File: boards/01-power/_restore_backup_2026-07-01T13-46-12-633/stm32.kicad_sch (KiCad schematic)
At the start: 26 parts, among them J3 TC2030, SW1 SW_BOOT, SW2 SW_BOOT, SW3 SW_BOOT, U3 STM32F405RGTx, Y1 16Mhz

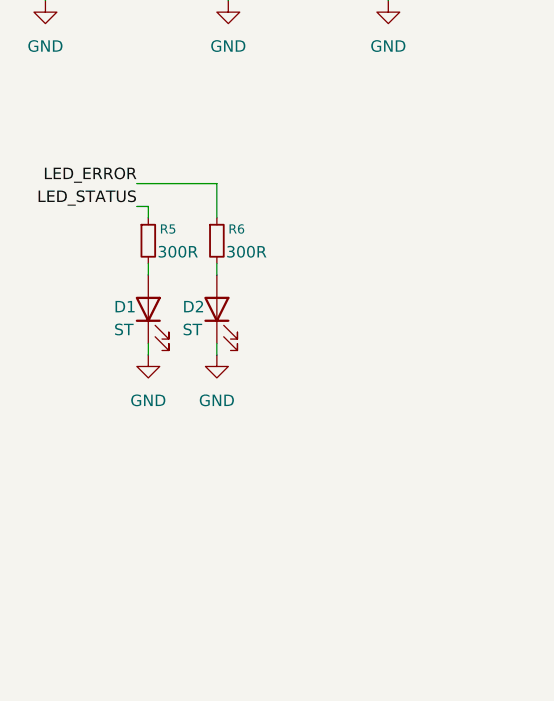
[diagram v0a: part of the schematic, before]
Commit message: chore: layout
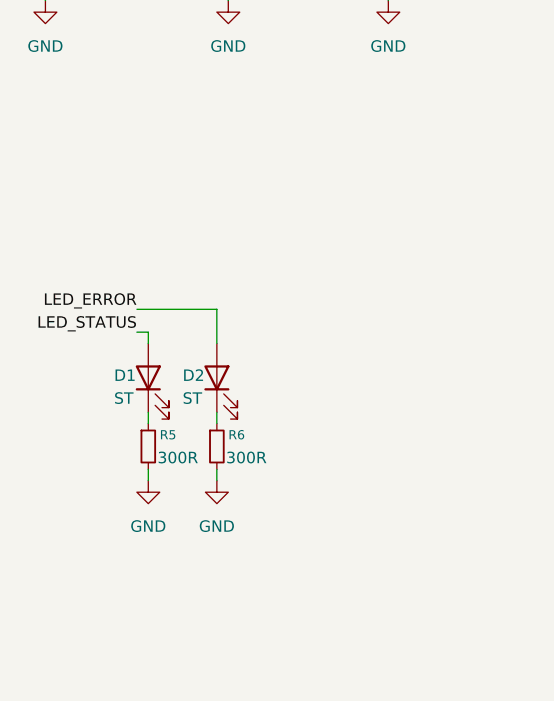
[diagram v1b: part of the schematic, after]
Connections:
- net GND: now also R5.2, R6.2; no longer D1.1 (K), D2.1 (K)
- net LED_ERROR: now also D2.2 (A); no longer R6.1
- net LED_STATUS: now also D1.2 (A); no longer R5.1
- new net: D1.1 (K), R5.1
- new net: D2.1 (K), R6.1
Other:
- moved on the sheet: D1, D2
